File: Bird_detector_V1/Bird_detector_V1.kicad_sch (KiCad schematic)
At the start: 0 parts

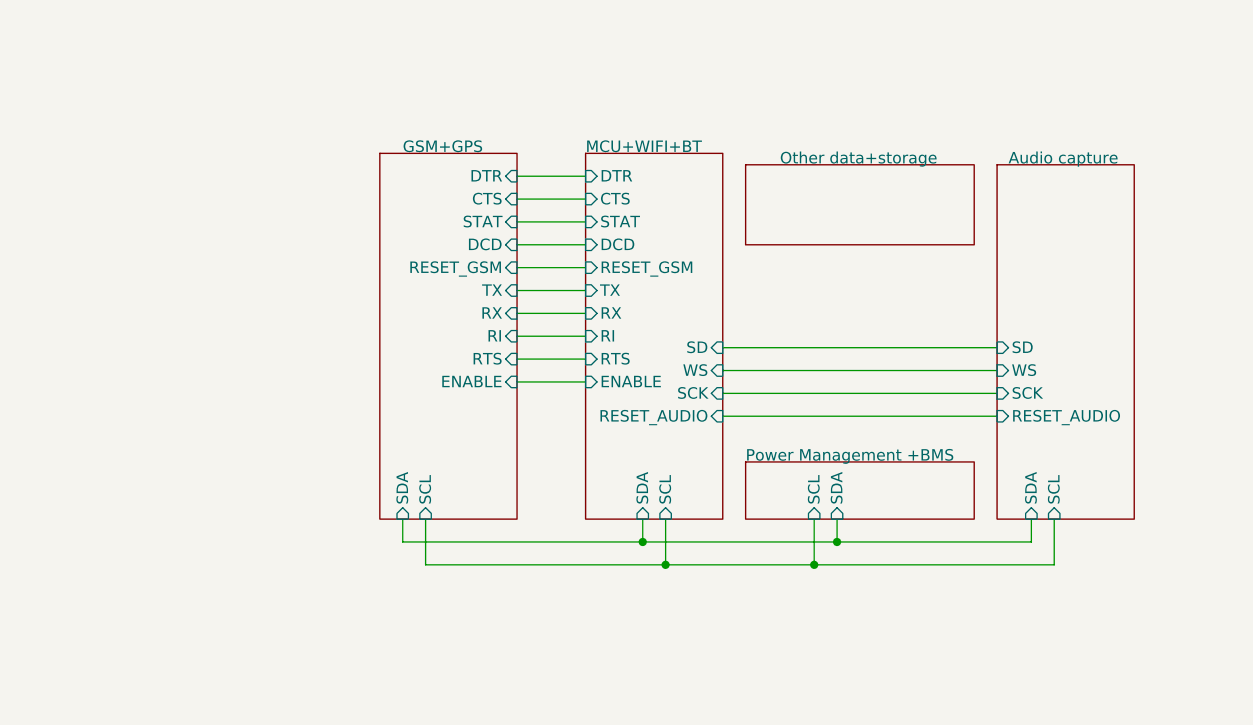
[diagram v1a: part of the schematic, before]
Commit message: f
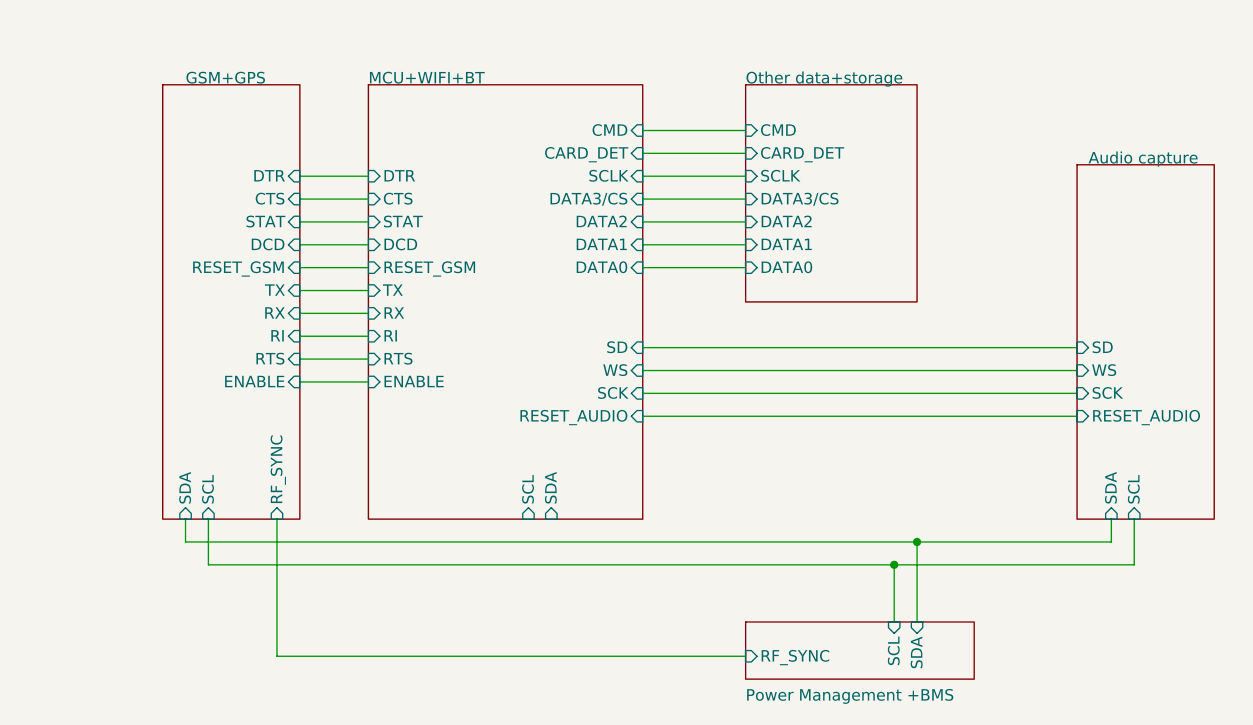
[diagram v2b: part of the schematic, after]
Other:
- sheet GSM+GPS ports: added RF_SYNC; removed none
- sheet MCU+WIFI+BT ports: added CARD_DET, CMD, DATA0, DATA1, DATA2, DATA3/CS, SCLK; removed none
- sheet Other data+storage ports: added CARD_DET, CMD, DATA0, DATA1, DATA2, DATA3/CS, SCLK; removed none
- sheet Power Management +BMS ports: added RF_SYNC; removed none
